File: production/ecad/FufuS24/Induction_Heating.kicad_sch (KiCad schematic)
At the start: 17 parts, among them J1 Conn_01x02, J14 691137710002, M1 MLX90614ESF-AAA-000-TU

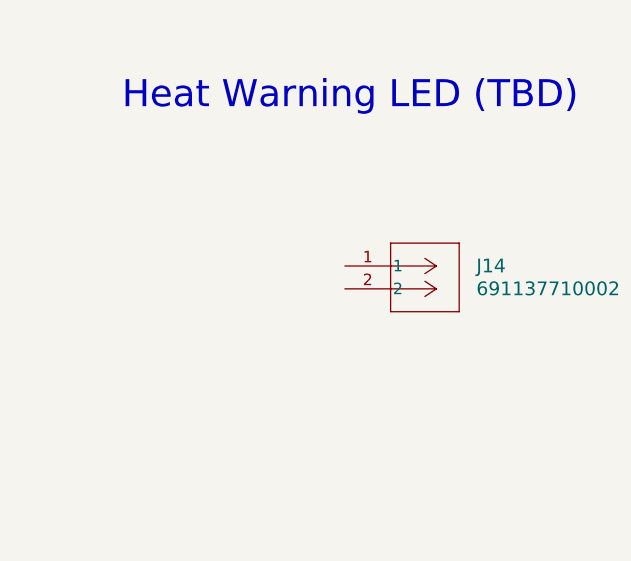
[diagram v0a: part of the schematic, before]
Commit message: efan 2
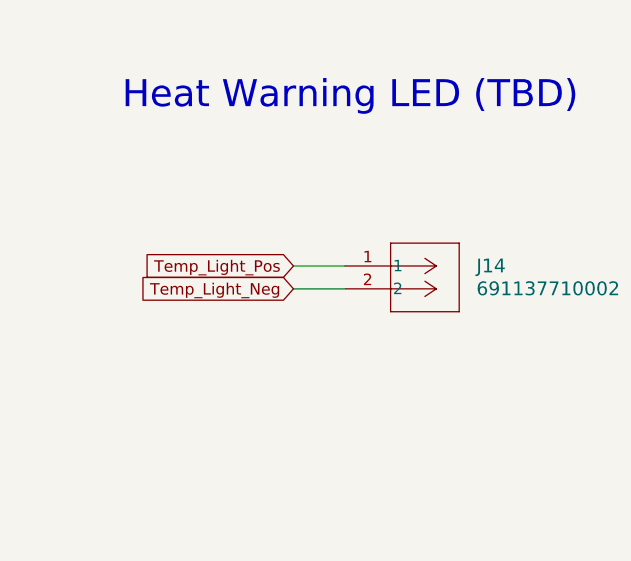
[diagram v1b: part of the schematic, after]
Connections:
- net Temp_Light_Pos: now reaches J14.1
- net Temp_Light_Neg: now reaches J14.2
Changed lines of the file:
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@@
+    (stroke (width 0) (type default))
+  )
+  (wire (pts (xy 41.91 41.275) (xy 47.625 41.275))
     (stroke (width 0) (type default))
   )
@@
     (stroke (width 0) (type default))
   )
+  (wire (pts (xy 41.91 38.735) (xy 47.625 38.735))
+    (stroke (width 0) (type default))
+  )
   (wire (pts (xy 49.53 147.32) (xy 55.88 147.32))
     (stroke (width 0) (type default))
@@
     (effects (font (size 1.27 1.27)) (justify left bottom))
   )
+  (global_label "Temp_Light_Neg" (shape input) (at 41.91 41.275 180) (fields_autoplaced)
+    (effects (font (size 1.27 1.27)) (justify right))
+    (property "Intersheetrefs" "${INTERSHEET_REFS}" (at 23.8664 41.275 0)
+      (effects (font (size 1.27 1.27)) (justify right) hide)
+    )
+  )
   (global_label "Heat_PWM1" (shape input) (at 26.67 138.43 180) (fields_autoplaced)
     (effects (font (size 1.27 1.27)) (justify right))
@@
     )
   )
+  (global_label "Temp_Light_Pos" (shape input) (at 41.91 38.735 180) (fields_autoplaced)
+    (effects (font (size 1.27 1.27)) (justify right))
+    (property "Intersheetrefs" "${INTERSHEET_REFS}" (at 23.9874 38.735 0)
+      (effects (font (size 1.27 1.27)) (justify right) hide)
+    )
+  )

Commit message: efan 3
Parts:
- C17: footprint footprints:U1-E_NCH -> footprints:CAPC2012X94N
- C18, C49: footprint 8600footprint:CAP_WCAP-ATG5_05.0X11.0_WRE -> footprints:CAPC2012X94N
- C4: footprint KiCad:ECQUAAF335LD -> footprints:CAPC2012X94N
- J14: footprint CONN2_710002_WRE -> footprints:CONN2_710002_WRE
- R11, R6, R7, R8: footprint (none) -> footprints:RESC2012X60N
- R9: footprint SQPfootprints:RES_SQP500_22X9P5_YAG -> footprints:RESC2012X60N
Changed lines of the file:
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@@
       (effects (font (size 1.524 1.524)) (justify left))
     )
-    (property "Footprint" "CONN2_710002_WRE" (at 47.625 38.735 0)
+    (property "Footprint" "footprints:CONN2_710002_WRE" (at 47.625 38.735 0)
       (effects (font (size 1.27 1.27) italic) hide)
     )
@@
       (effects (font (size 1.27 1.27)))
     )
-    (property "Footprint" "" (at 122.174 161.036 90)
+    (property "Footprint" "footprints:RESC2012X60N" (at 122.174 161.036 90)
       (effects (font (size 1.27 1.27)) hide)
     )
@@
       (effects (font (size 1.27 1.27)) (justify left))
     )
-    (property "Footprint" "footprints:U1-E_NCH" (at 83.82 118.11 0)
+    (property "Footprint" "footprints:CAPC2012X94N" (at 83.82 118.11 0)
       (effects (font (size 1.27 1.27) italic) hide)
     )
@@
       (effects (font (size 1.27 1.27)) (justify left))
     )
-    (property "Footprint" "SQPfootprints:RES_SQP500_22X9P5_YAG" (at 106.68 160.02 0)
+    (property "Footprint" "footprints:RESC2012X60N" (at 106.68 160.02 0)
       (effects (font (size 1.27 1.27) italic) hide)
     )
@@
       (effects (font (size 1.27 1.27)) (justify left))
     )
-    (property "Footprint" "8600footprint:CAP_WCAP-ATG5_05.0X11.0_WRE" (at 132.08 165.1 0)
+    (property "Footprint" "footprints:CAPC2012X94N" (at 132.08 165.1 0)
       (effects (font (size 1.27 1.27) italic) hide)
     )
@@
       (effects (font (size 1.27 1.27)))
     )
-    (property "Footprint" "" (at 39.624 137.414 90)
+    (property "Footprint" "footprints:RESC2012X60N" (at 39.624 137.414 90)
       (effects (font (size 1.27 1.27)) hide)
     )
@@
       (effects (font (size 1.27 1.27)))
     )
-    (property "Footprint" "" (at 87.249 137.414 90)
+    (property "Footprint" "footprints:RESC2012X60N" (at 87.249 137.414 90)
       (effects (font (size 1.27 1.27)) hide)
     )
@@
       (effects (font (size 1.27 1.27)))
     )
-    (property "Footprint" "KiCad:ECQUAAF335LD" (at 149.86 178.74 0)
+    (property "Footprint" "footprints:CAPC2012X94N" (at 149.86 178.74 0)
       (effects (font (size 1.27 1.27)) (justify left top) hide)
     )
@@
       (effects (font (size 1.27 1.27)) (justify left))
     )
-    (property "Footprint" "8600footprint:CAP_WCAP-ATG5_05.0X11.0_WRE" (at 257.81 95.25 0)
+    (property "Footprint" "footprints:CAPC2012X94N" (at 257.81 95.25 0)
       (effects (font (size 1.27 1.27) italic) hide)
     )
@@
       (effects (font (size 1.27 1.27)) (justify right))
     )
-    (property "Footprint" "" (at 91.694 148.336 90)
-      (effects (font (size 1.27 1.27)) hide)
-    )
+    (property "Footprint" "footprints:RESC2012X60N" (at 91.694 148.336 90)
+      (effects (font (size 1.27 1.27)) hide)
+    )

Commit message: efan 5
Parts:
- J1: footprint B2B-XH-A_LF__SN_:JST_B2B-XH-A_LF__SN_ -> footprints:CON_5025840270_MOL
- TP9: footprint TestPoint:TestPoint_Pad_2.0x2.0mm -> footprints:TP_5014
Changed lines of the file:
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@@
       (effects (font (size 1.27 1.27)) (justify left))
     )
-    (property "Footprint" "TestPoint:TestPoint_Pad_2.0x2.0mm" (at 135.89 165.1 0)
+    (property "Footprint" "footprints:TP_5014" (at 135.89 165.1 0)
       (effects (font (size 1.27 1.27)) hide)
     )
@@
       (effects (font (size 1.27 1.27)))
     )
-    (property "Footprint" "B2B-XH-A_LF__SN_:JST_B2B-XH-A_LF__SN_" (at 123.19 104.14 0)
+    (property "Footprint" "footprints:CON_5025840270_MOL" (at 123.19 104.14 0)
       (effects (font (size 1.27 1.27)) hide)
     )
